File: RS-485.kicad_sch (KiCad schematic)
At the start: 7 parts, among them J10 RJ45, J11 Conn_01x03, J12 Conn_01x04, J16 Conn_01x04, U2 SP3485CN

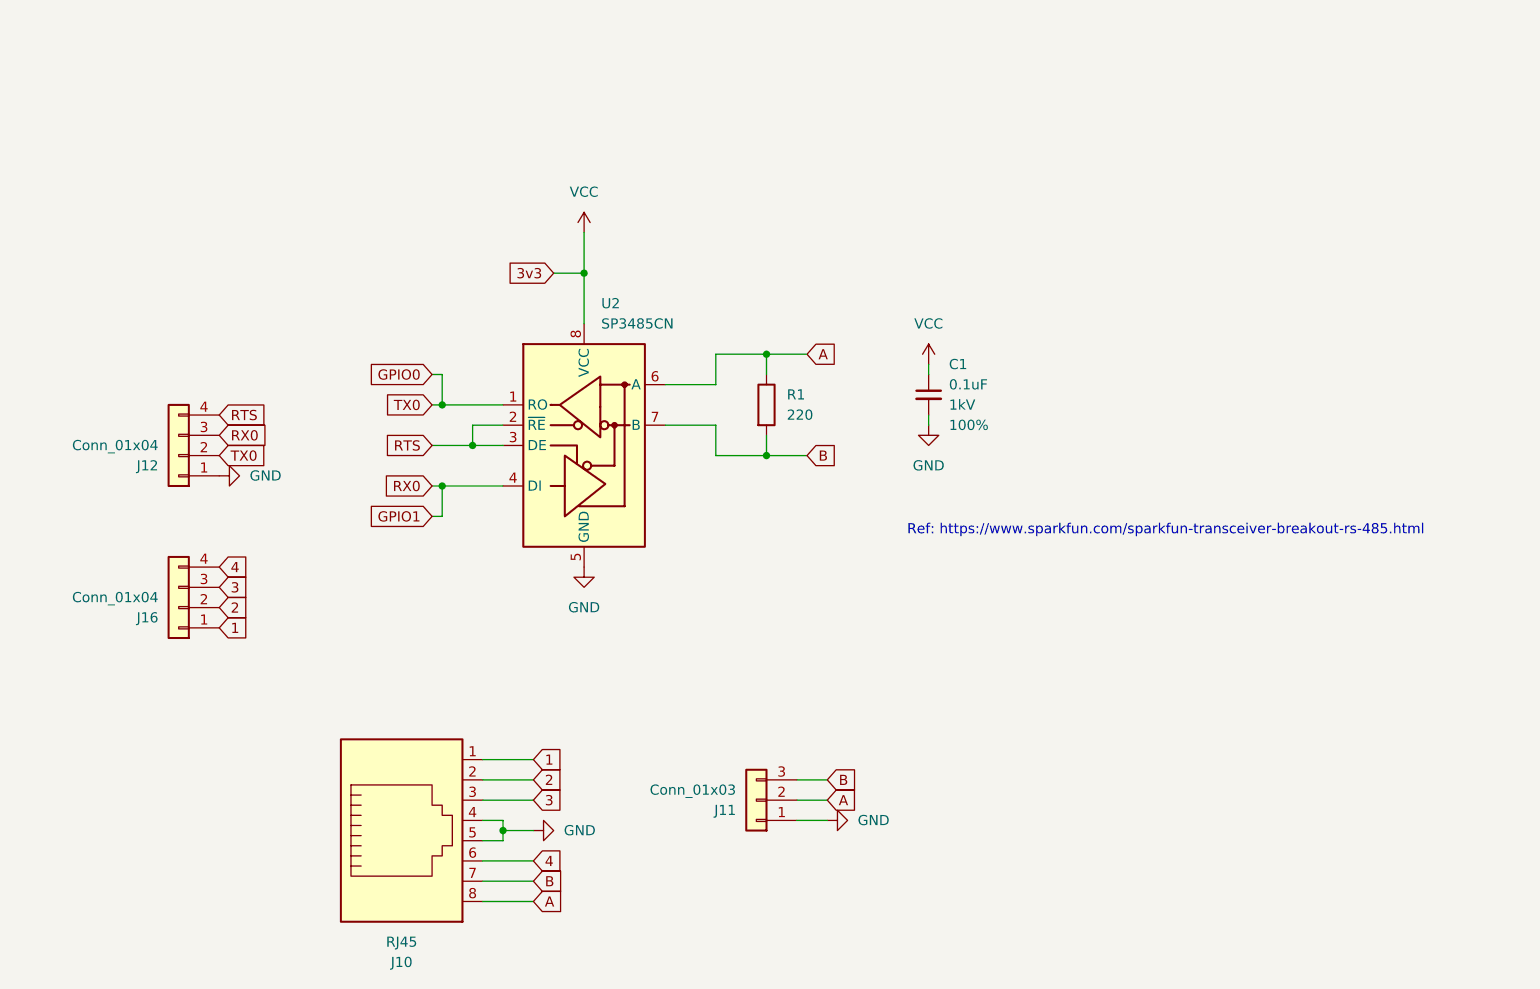
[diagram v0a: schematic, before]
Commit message: updated schematics etc
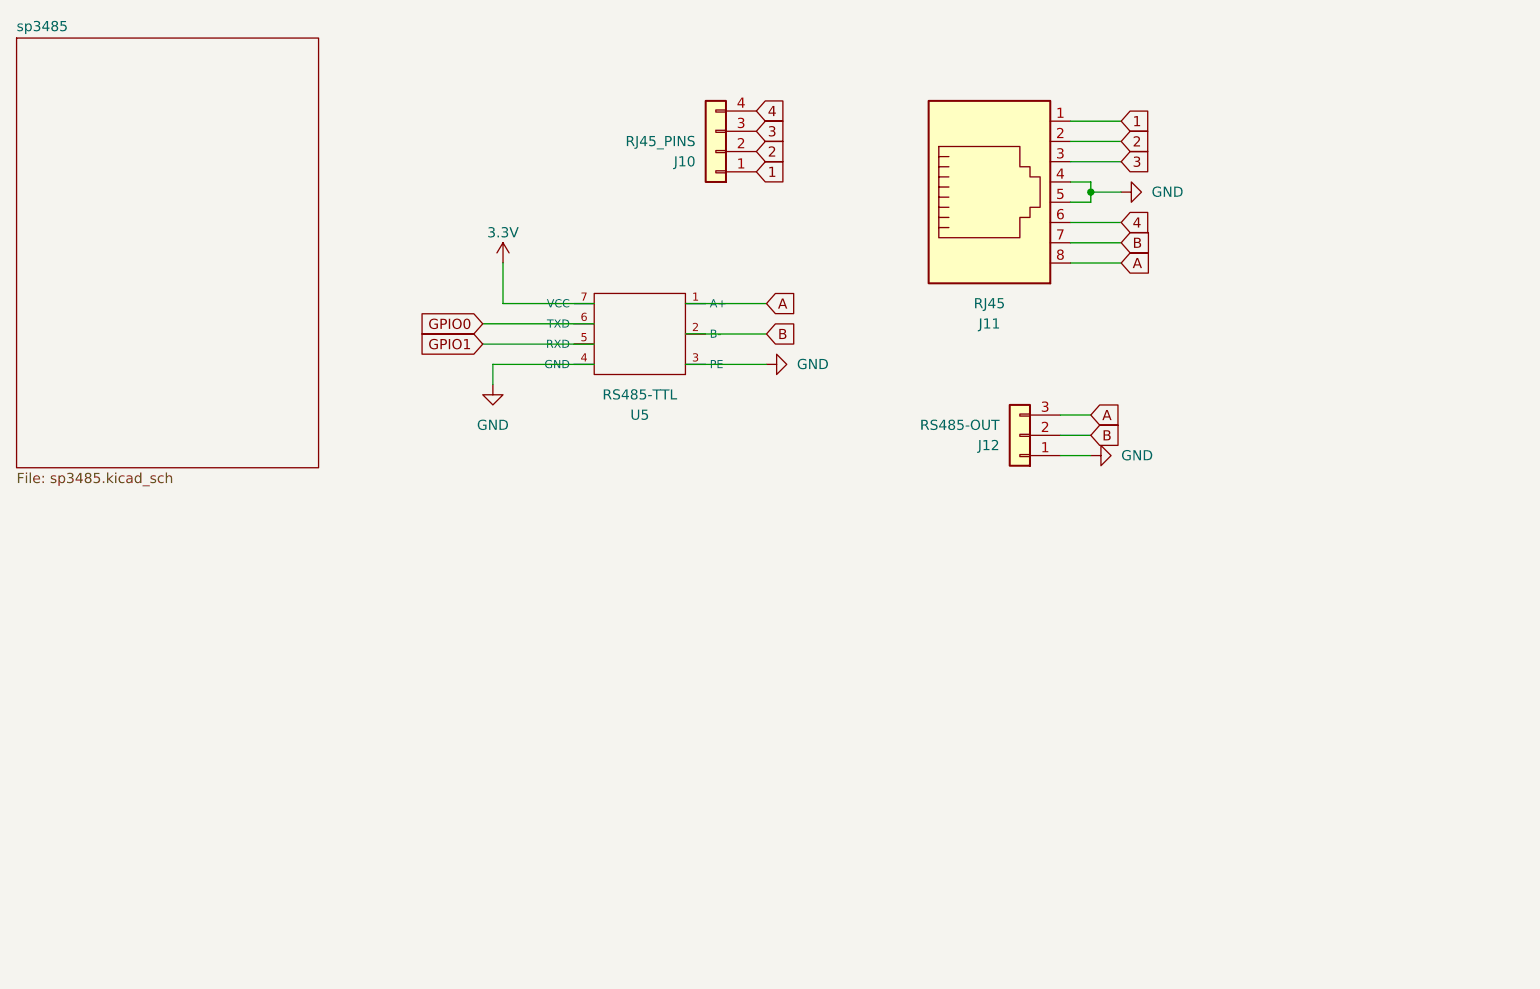
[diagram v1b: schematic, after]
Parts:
- removed C1: 0.1uF, SparkFun-Capacitor:C_0603_1608Metric, symbol SparkFun-Capacitor:C
- removed J12: Conn_01x04, symbol Connector_Generic:Conn_01x04
- removed R1: 220, Resistor_SMD:R_0603_1608Metric, symbol Device:R
- removed U2: SP3485CN, Package_SO:SOIC-8_3.9x4.9mm_P1.27mm, symbol Interface_UART:SP3485CN
- added U5: RS485-TTL, Waveshare-TTL-To-RS485-C-Kicad:Waveshare-RS485-TTL, symbol waveshare-rs485-ttl:waveshare-rs485-ttl
- J10: renamed from J16; value Conn_01x04 -> RJ45_PINS; footprint (none) -> Connector_PinHeader_2.54mm:PinHeader_1x04_P2.54mm_Vertical
- J12: renamed from J11; value Conn_01x03 -> RS485-OUT; footprint (none) -> Connector_Phoenix_MC:PhoenixContact_MC_1,5_3-G-3.81_1x03_P3.81mm_Horizontal
- renumbered J10 to J11
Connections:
- net A: now also J12.3 (Pin_3), U5.1 (A+); no longer J12.2 (Pin_2)
- net B: now also J12.2 (Pin_2), U5.2 (B-); no longer J12.3 (Pin_3)
- net GND: now also U5.3 (PE), U5.4 (GND)
- net GPIO0: now also U5.6 (TXD)
- net GPIO1: now also U5.5 (RXD)
- new net 3.3V: U5.7 (VCC)
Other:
- added sheet sp3485 (sp3485.kicad_sch)
- note removed: "Ref: https://www.sparkfun.com/sparkfun-transceiver-breakout-rs-485.html"
- moved on the sheet: J10, J11, J12
